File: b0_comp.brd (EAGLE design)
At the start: 93 x 70 mm, 1 part

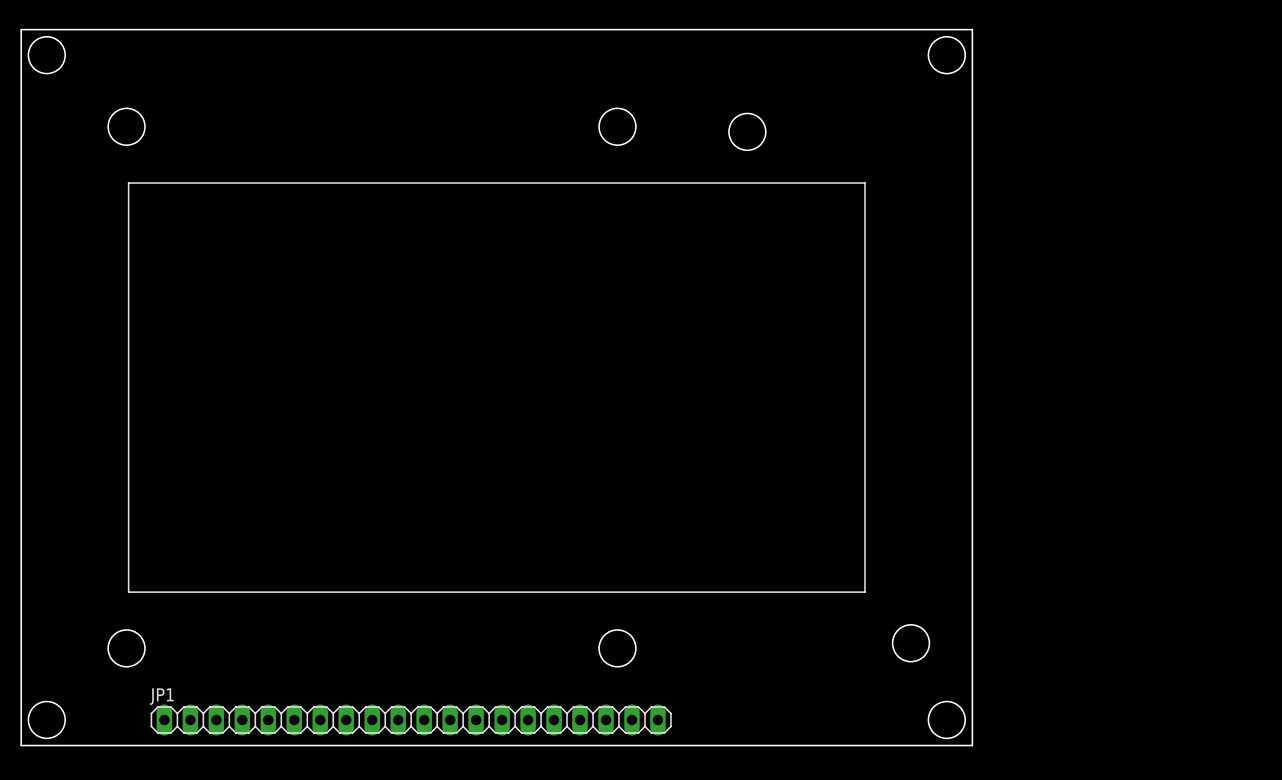
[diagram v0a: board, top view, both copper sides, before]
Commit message: .
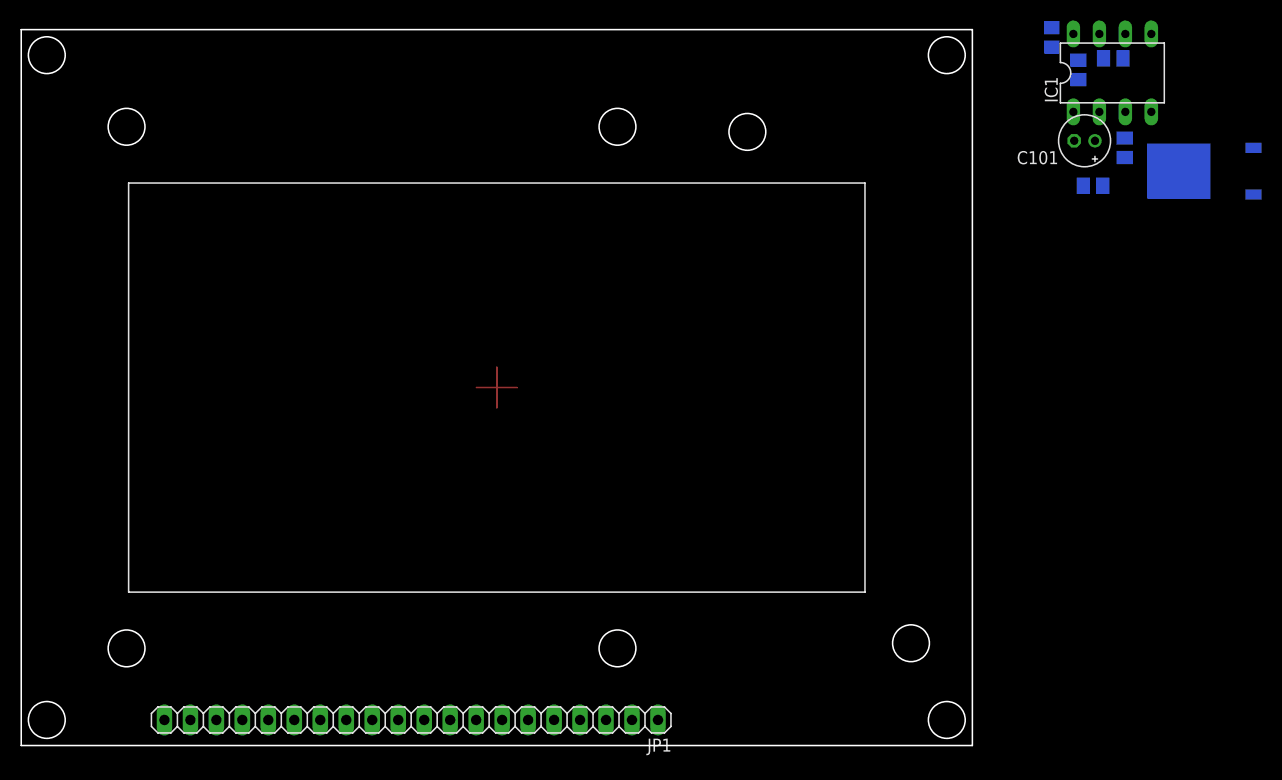
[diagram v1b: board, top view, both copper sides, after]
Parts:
- added C101: 4m7, rcl:E2-5
- added C102: 100n, rcl:C0805
- added IC1: КР1016ВИ1(NE555), st-microelectronics:DIL-08
- added R101*, R101*1: 22k, rcl:M0805
- added R102*: 180k, rcl:M0805
- added R103: 2k2, rcl:M0805
- added VT1: (no value), m_transistor:DPACK
- turned JP1 to 180 degrees
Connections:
- new net +12V: VT1.D
- new net GND: R101*1.1
- new net N$1: JP1.19, JP1.20
- new net N$4: IC1.7, R101*.1, R102*.2
- new net N$5: C101.+, IC1.2, IC1.6, R102*.1
- new net N$6: C102.1, IC1.5
- new net N$7: IC1.3, R103.1
- new net N$8: R103.2, VT1.G
- new net VCC/2: IC1.4, IC1.8, R101*.2
- new net VSS: C101.-, C102.2, IC1.1, R101*1.2, VT1.S
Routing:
- net N$3: track 0.00 -> 4.00 mm
- net N$2: track 0.00 -> 4.00 mm
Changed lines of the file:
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@@
 <setting verticaltext="up"/>
 </settings>
-<grid distance="9.84251969" unitdist="mil" unit="mil" style="lines" multiple="1" display="yes" altdistance="0.025" altunitdist="inch" altunit="inch"/>
+<grid distance="25" unitdist="mil" unit="mil" style="lines" multiple="1" display="yes" altdistance="0.025" altunitdist="inch" altunit="inch"/>
 <layers>
 <layer number="1" name="Top" color="4" fill="1" visible="yes" active="yes"/>
@@
 <layer number="56" name="wert" color="7" fill="1" visible="no" active="no"/>
 <layer number="57" name="tCAD" color="7" fill="1" visible="no" active="no"/>
+<layer number="90" name="Modules" color="7" fill="1" visible="yes" active="yes"/>
 <layer number="91" name="Nets" color="2" fill="1" visible="no" active="no"/>
 <layer number="92" name="Busses" color="1" fill="1" visible="no" active="no"/>
@@
 <layer number="112" name="tSilk" color="7" fill="1" visible="no" active="yes"/>
 <layer number="113" name="ReferenceLS" color="7" fill="1" visible="no" active="no"/>
+<layer number="114" name="bJumper" color="7" fill="1" visible="yes" active="yes"/>
+<layer number="115" name="GND" color="7" fill="1" visible="yes" active="yes"/>
 <layer number="116" name="Patch_BOT" color="9" fill="4" visible="no" active="yes"/>
+<layer number="117" name="tJumper" color="7" fill="1" visible="yes" active="yes"/>
 <layer number="118" name="Rect_Pads" color="7" fill="1" visible="no" active="no"/>
 <layer number="121" name="_tsilk" color="7" fill="1" visible="no" active="yes"/>
@@
 <layer number="251" name="SMDround" color="7" fill="1" visible="no" active="no"/>
 <layer number="254" name="cooling" color="7" fill="1" visible="no" active="yes"/>
+<layer number="255" name="routoute" color="7" fill="1" visible="yes" active="yes"/>
 </layers>
 <board>
@@
 </autorouter>
 <elements>
-<element name="JP1" library="Разъёмы штырьковые 2.54мм" package="1X20" value="" x="-8.371840625" y="-32.50438125"/>
+<element name="JP1" library="Разъёмы штырьковые 2.54мм" package="1X20" value="" x="-8.37" y="-32.5" rot="R180"/>
+<element name="IC1" library="st-microelectronics" package="DIL-08" value="КР1016ВИ1(NE555)" x="60.185" y="30.765">
+<attribute name="OC_NEWARK" value="89K1486" x="60.185" y="30.765" size="1.778" layer="27" display="off"/>
+<attribute name="MPN" value="NE555N" x="60.185" y="30.765" size="1.778" layer="27" display="off"/>
+<attribute name="MF" value="Arrow Electronics" x="60.185" y="30.765" size="1.778" layer="27" display="off"/>
+<attribute name="OC_FARNELL" value="1467742" x="60.185" y="30.765" size="1.778" layer="27" display="off"/>
+</element>
+<element name="R102*" library="rcl" package="M0805" value="180k" x="60.275" y="32.185" rot="MR0"/>
+<element name="R101*" library="rcl" package="M0805" value="22k" x="56.865" y="31.065" rot="MR270"/>
+<element name="C101" library="rcl" package="E2-5" value="4m7" x="57.47" y="24.13" rot="R180"/>
+<element name="C102" library="rcl" package="C0805" value="100n" x="54.26" y="34.24" rot="MR270"/>
+<element name="R103" library="rcl" package="M0805" value="2k2" x="61.395" y="23.445" rot="MR270"/>
+<element name="VT1" library="m_transistor" package="DPACK" value="" x="69.19" y="21.16" rot="MR270"/>
+<element name="R101*1" library="rcl" package="M0805" value="22k" x="58.3" y="19.735" rot="MR0"/>
 </elements>
 <signals>
+<signal name="N$2">
+<wire x1="0" y1="2" x2="0" y2="-2" width="0.1524" layer="1"/>
+</signal>
+<signal name="N$3">
+<wire x1="-2" y1="0" x2="2" y2="0" width="0.1524" layer="1"/>
+</signal>
+<signal name="N$1">
+<contactref element="JP1" pad="20"/>
+<contactref element="JP1" pad="19"/>
+<wire x1="-29.96" y1="-32.5" x2="-32.5" y2="-32.5" width="0" layer="19" extent="1-1"/>
+</signal>
+<signal name="N$5">
+<contactref element="IC1" pad="2"/>
+<contactref element="IC1" pad="6"/>
+<contactref element="R102*" pad="1"/>
+<contactref element="C101" pad="+"/>
+<wire x1="61.225" y1="32.185" x2="61.455" y2="34.575" width="0" layer="19" extent="16-16"/>
+<wire x1="58.915" y1="26.955" x2="61.225" y2="32.185" width="0" layer="19" extent="16-16"/>
+<wire x1="58.486" y1="24.13" x2="58.915" y2="26.955" width="0" layer="19" extent="1-1"/>
+</signal>
+<signal name="N$4">
+<contactref element="R102*" pad="2"/>
+<contactref element="IC1" pad="7"/>
+<contactref element="R101*" pad="1"/>
+<wire x1="59.325" y1="32.185" x2="58.915" y2="34.575" width="0" layer="19" extent="16-16"/>
+<wire x1="56.865" y1="32.015" x2="59.325" y2="32.185" width="0" layer="19" extent="16-16"/>
+</signal>
+<signal name="N$6">
+<contactref element="IC1" pad="5"/>
+<contactref element="C102" pad="1"/>
+<wire x1="54.26" y1="35.19" x2="63.995" y2="34.575" width="0" layer="19" extent="16-16"/>
+</signal>
+<signal name="N$7">
+<contactref element="IC1" pad="3"/>
+<contactref element="R103" pad="1"/>
+<wire x1="61.395" y1="24.395" x2="61.455" y2="26.955" width="0" layer="19" extent="16-16"/>
+</signal>
+<signal name="N$8">
+<contactref element="R103" pad="2"/>
+<contactref element="VT1" pad="G"/>
+<wire x1="61.395" y1="22.495" x2="73.99" y2="23.44" width="0" layer="19" extent="16-16"/>
+</signal>
+<signal name="GND">
+<contactref element="R101*1" pad="1"/>
+</signal>
+<signal name="+12V">
+<contactref element="VT1" pad="D"/>
+</signal>
+<signal name="VSS">
+<contactref element="IC1" pad="1"/>
+<contactref element="C101" pad="-"/>
+<contactref element="C102" pad="2"/>
+<contactref element="VT1" pad="S"/>
+<contactref element="R101*1" pad="2"/>
+<wire x1="56.375" y1="26.955" x2="54.26" y2="33.29" width="0" layer="19" extent="16-16"/>
+<wire x1="56.454" y1="24.13" x2="56.375" y2="26.955" width="0" layer="19" extent="1-1"/>
+<wire x1="57.35" y1="19.735" x2="56.454" y2="24.13" width="0" layer="19" extent="16-16"/>
+<wire x1="73.99" y1="18.88" x2="57.35" y2="19.735" width="0" layer="19" extent="16-16"/>
+</signal>
+<signal name="VCC/2">
+<contactref element="IC1" pad="4"/>
+<contactref element="IC1" pad="8"/>
+<contactref element="R101*" pad="2"/>
+<wire x1="56.865" y1="30.115" x2="63.995" y2="26.955" width="0" layer="19" extent="16-16"/>
+<wire x1="56.375" y1="34.575" x2="56.865" y2="30.115" width="0" layer="19" extent="16-16"/>
+</signal>
 </signals>
 </board>
